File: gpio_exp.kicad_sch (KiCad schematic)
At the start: 23 parts, among them U11 MCP23S17_SO

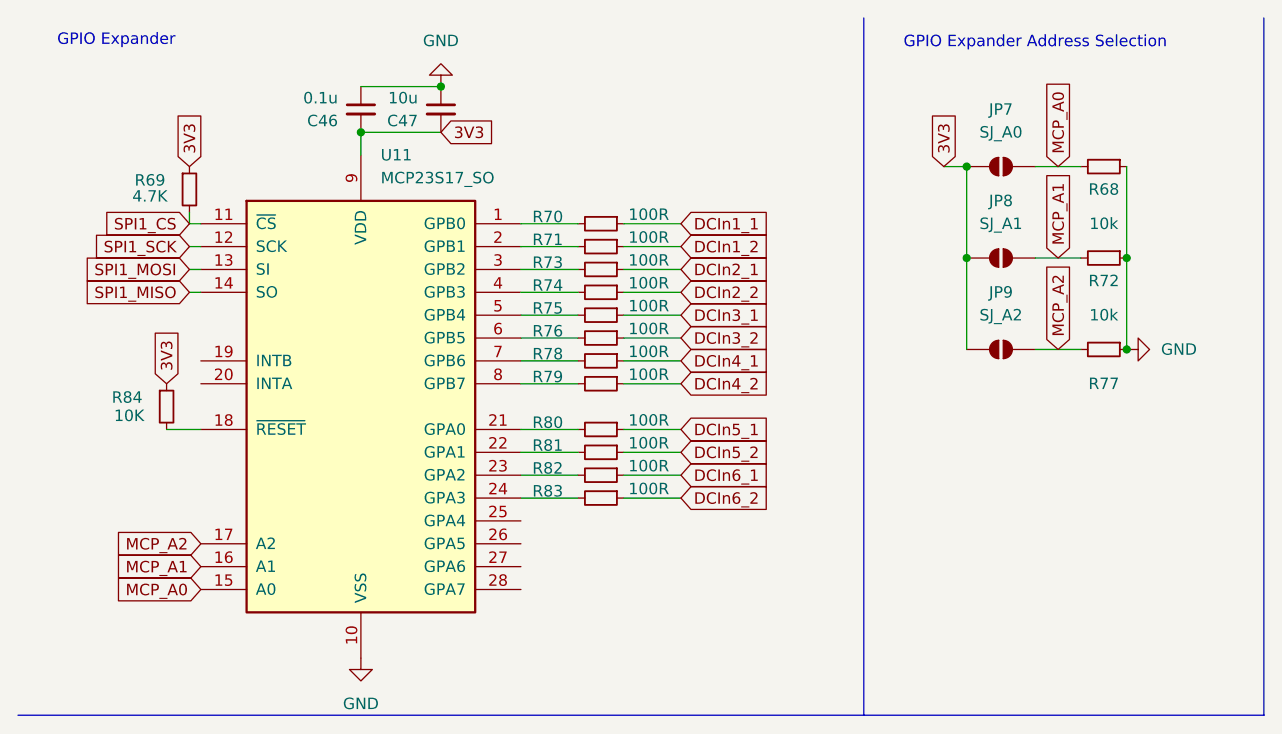
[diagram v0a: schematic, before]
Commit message: dc sürücü yol çizimleri yapıldı
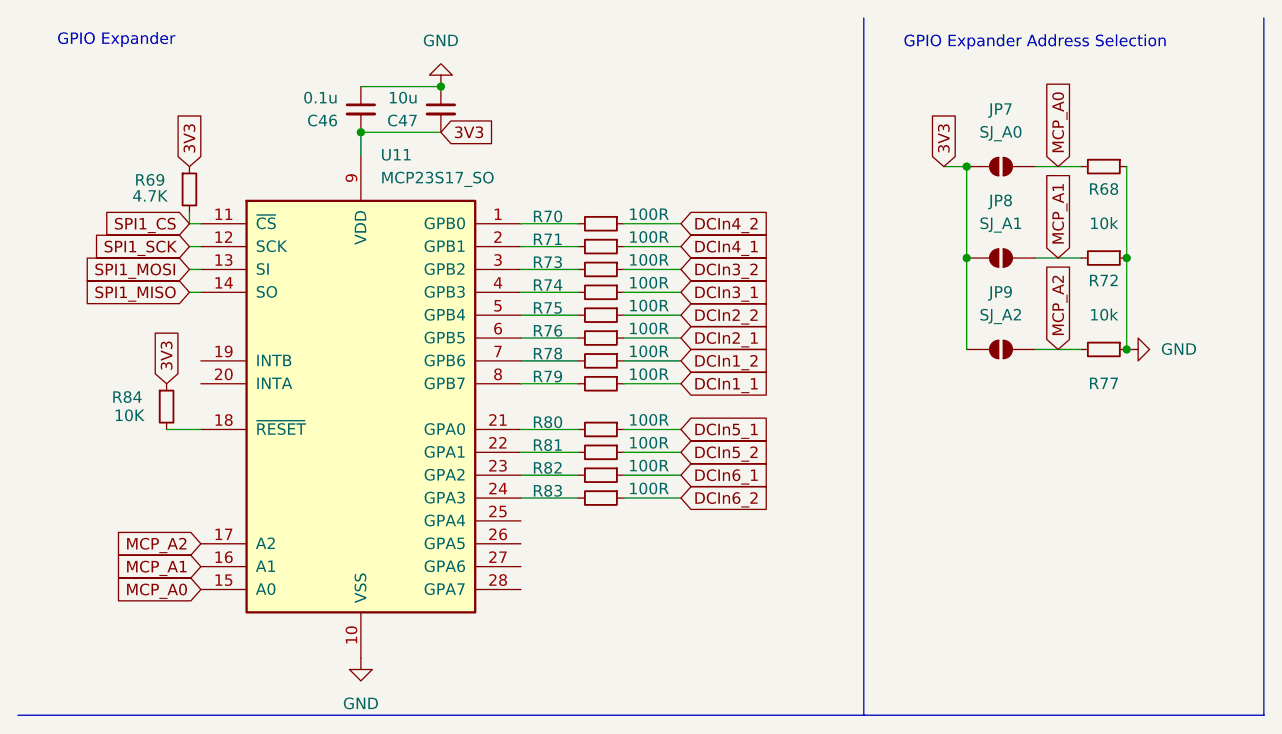
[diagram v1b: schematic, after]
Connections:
- net DCIn1_1: now also R79.1; no longer R70.1
- net DCIn1_2: now also R78.1; no longer R71.1
- net DCIn2_1: now also R76.1; no longer R73.1
- net DCIn2_2: now also R75.1; no longer R74.1
- net DCIn3_1: now also R74.1; no longer R75.1
- net DCIn3_2: now also R73.1; no longer R76.1
- net DCIn4_1: now also R71.1; no longer R78.1
- net DCIn4_2: now also R70.1; no longer R79.1

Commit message: Routing
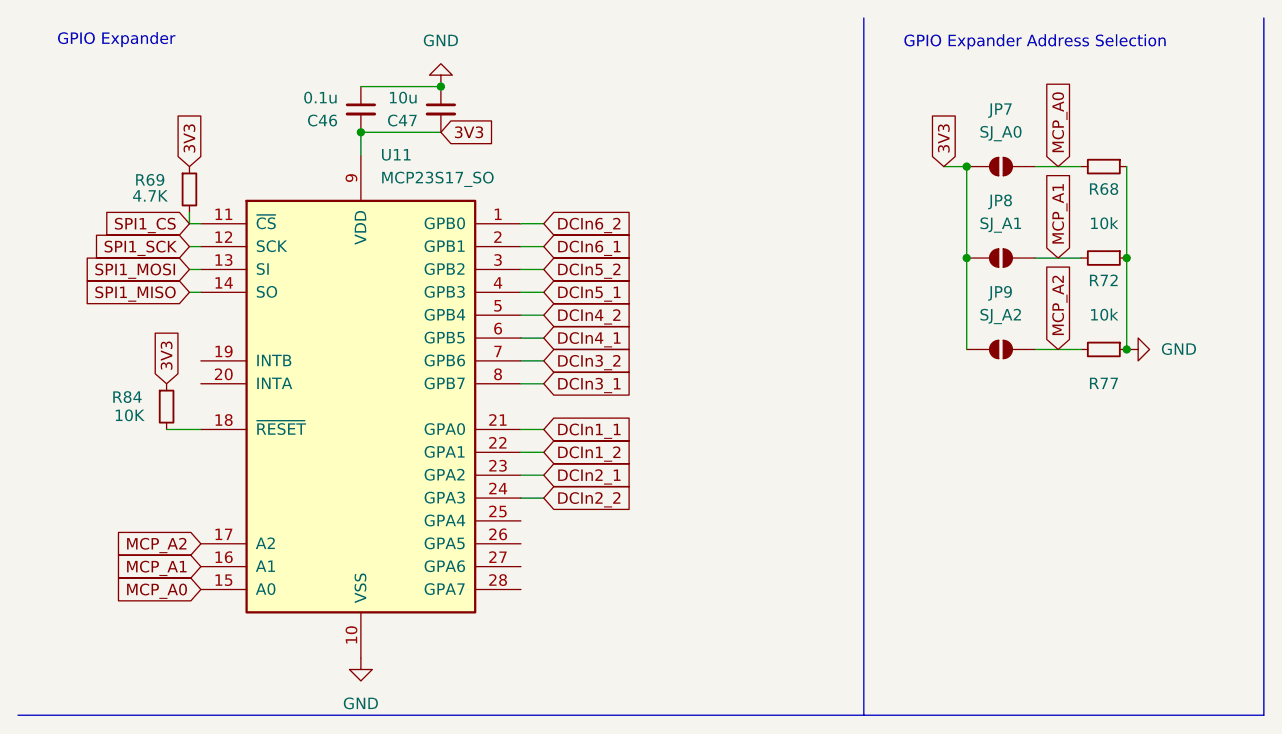
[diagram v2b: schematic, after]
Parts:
- removed R70, R71, R73, R74, R75, R76, R78, R79, R80, R81, R82, R83: 100R, Resistor_SMD:R_0805_2012Metric, symbol Device:R_Small
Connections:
- net DCIn1_1: now also U11.21 (GPA0)
- net DCIn1_2: now also U11.22 (GPA1)
- net DCIn2_1: now also U11.23 (GPA2)
- net DCIn2_2: now also U11.24 (GPA3)
- net DCIn3_1: now also U11.8 (GPB7)
- net DCIn3_2: now also U11.7 (GPB6)
- net DCIn4_1: now also U11.6 (GPB5)
- net DCIn4_2: now also U11.5 (GPB4)
- net DCIn5_1: now also U11.4 (GPB3)
- net DCIn5_2: now also U11.3 (GPB2)
- net DCIn6_1: now also U11.2 (GPB1)
- net DCIn6_2: now also U11.1 (GPB0)
